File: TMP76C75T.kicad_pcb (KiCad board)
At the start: 2 copper layers, 116.8 x 91.4 mm, 54 parts, among them J1 Conn_01x08_Male, J2 Conn_01x07_Male, J3 Conn_01x08_Male, J3-2 Conn_01x08_Male, J4 Conn_01x08_Male, J4-2 Conn_01x08_Male, J4-ADDR1 Conn_01x08_Male, J5 Conn_01x08_Male, J6 Conn_01x06_Male, J7 Conn_01x08_Male, SW1 SW_DIP_x03, SW2 SW_Push_SPDT, U1 TMP76C75T, U2 27C256, U3 M60011-0131J, U4 LM78M05_TO220

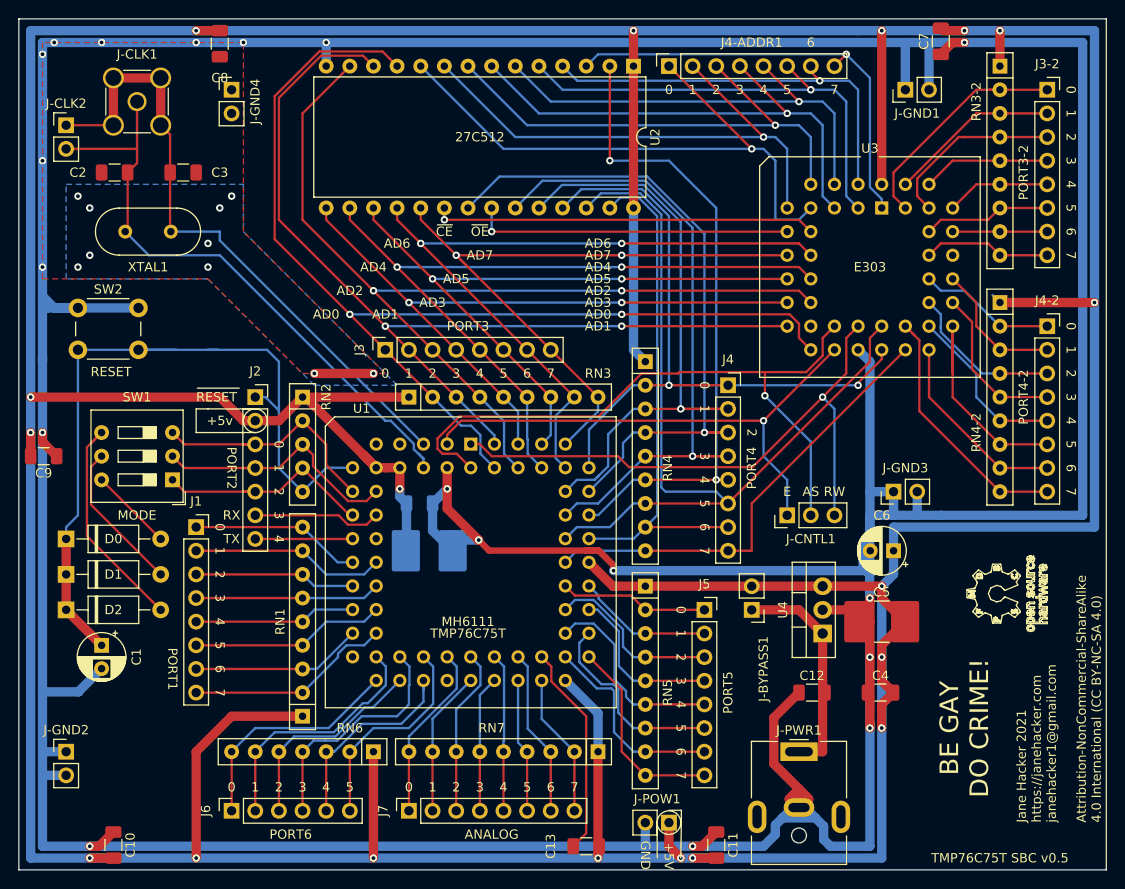
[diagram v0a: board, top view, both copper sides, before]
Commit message: Updates
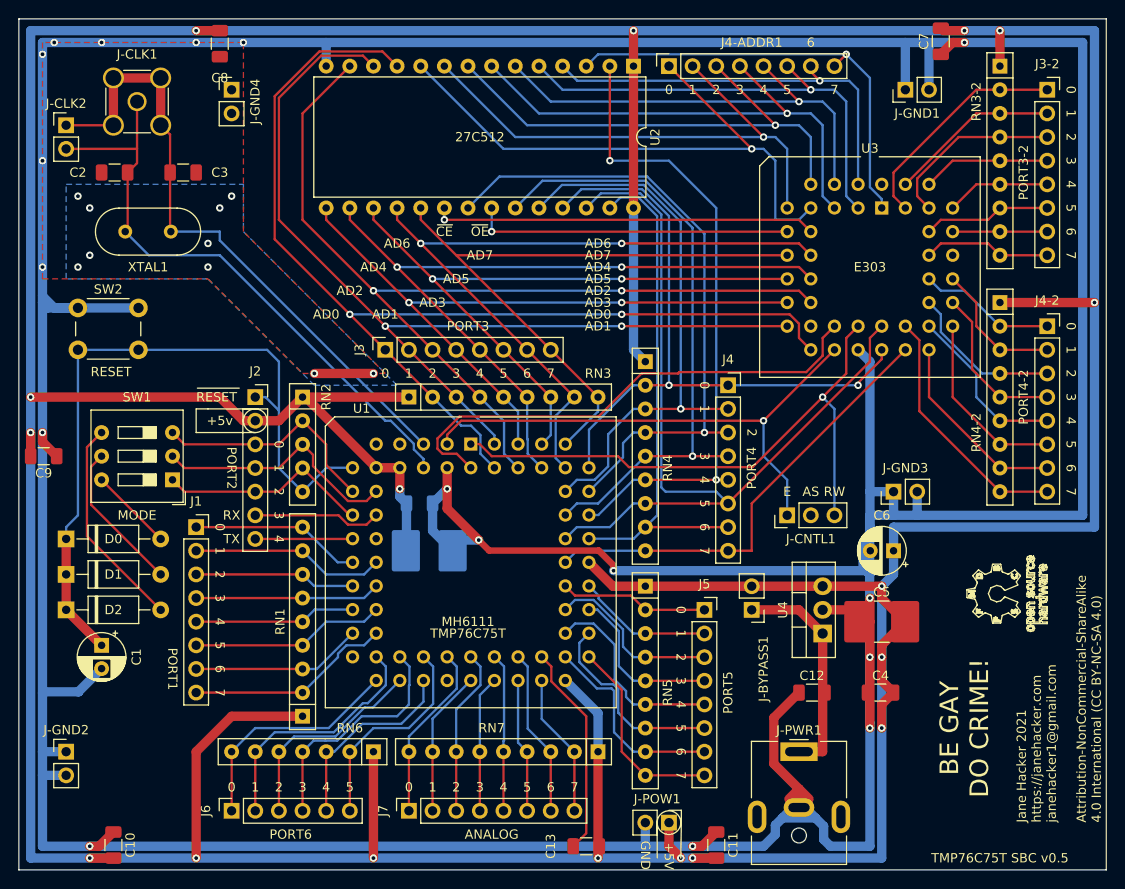
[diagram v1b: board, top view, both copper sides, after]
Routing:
- net +5V: track 689.3 -> 666.3 mm, vias 18 -> 17
- net /AS: track 72.0 -> 54.3 mm, vias 1 -> 0
- net GND: track 684.6 -> 678.7 mm, vias 28 -> 27
- net /A9: track 66.6 -> 61.2 mm
- net /RESET: track 85.7 -> 80.6 mm
- net /P4.5: track 25.0 -> 19.9 mm
- net /A11: track 70.8 -> 67.0 mm
- net /VIN: track 26.5 -> 23.9 mm
- net /A10: track 71.7 -> 69.2 mm
- net /P2.2: track 24.6 -> 22.7 mm
- net /AD7: track 72.1 -> 70.3 mm, vias 2 -> 0
- net Net-(D2-Pad2): track 24.6 -> 23.0 mm
- net /P4.7: track 28.5 -> 27.1 mm
- net /P2.1: track 28.4 -> 27.1 mm
- net /P2.0: track 26.6 -> 25.4 mm
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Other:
- net class Default removed
